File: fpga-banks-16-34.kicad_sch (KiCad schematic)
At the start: 25 parts, among them U1 ASFLMB-100.000MHZ-XY-T, U15 XC7K160T-FFG676, U8 PCA9517ADMR2G

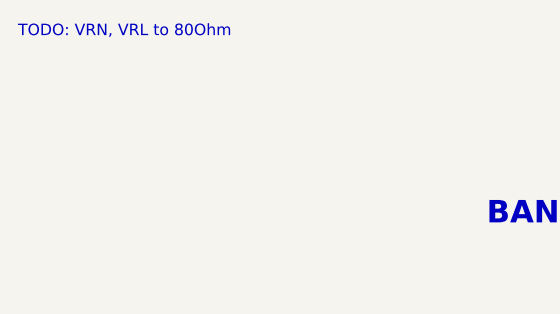
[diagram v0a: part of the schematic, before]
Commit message: SI improvments
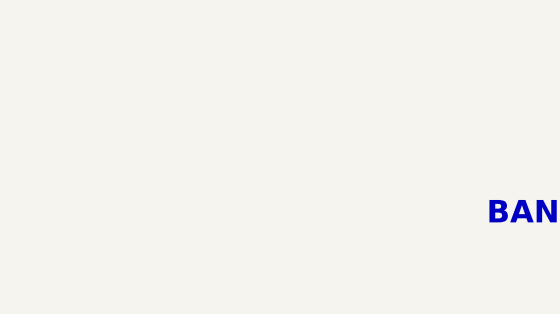
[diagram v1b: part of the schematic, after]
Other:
- note removed: "TODO: VRN, VRL to 80Ohm"
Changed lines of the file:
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@@
     (effects (font (size 2.4892 2.4892) (thickness 0.4978) bold) (justify left bottom))
-  )
-  (text "TODO: VRN, VRL to 80Ohm\n" (at 1.905 3.81 0)
-    (effects (font (size 1.27 1.27)) (justify left bottom))
   )
   (global_label "DQ51" (shape input) (at 165.735 157.48 0) (fields_autoplaced)
